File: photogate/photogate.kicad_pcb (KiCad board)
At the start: 2 copper layers, 72.8 x 62.1 mm, 21 parts, among them P2 3poles LOGO, P2 Jack F SJ1-3525N

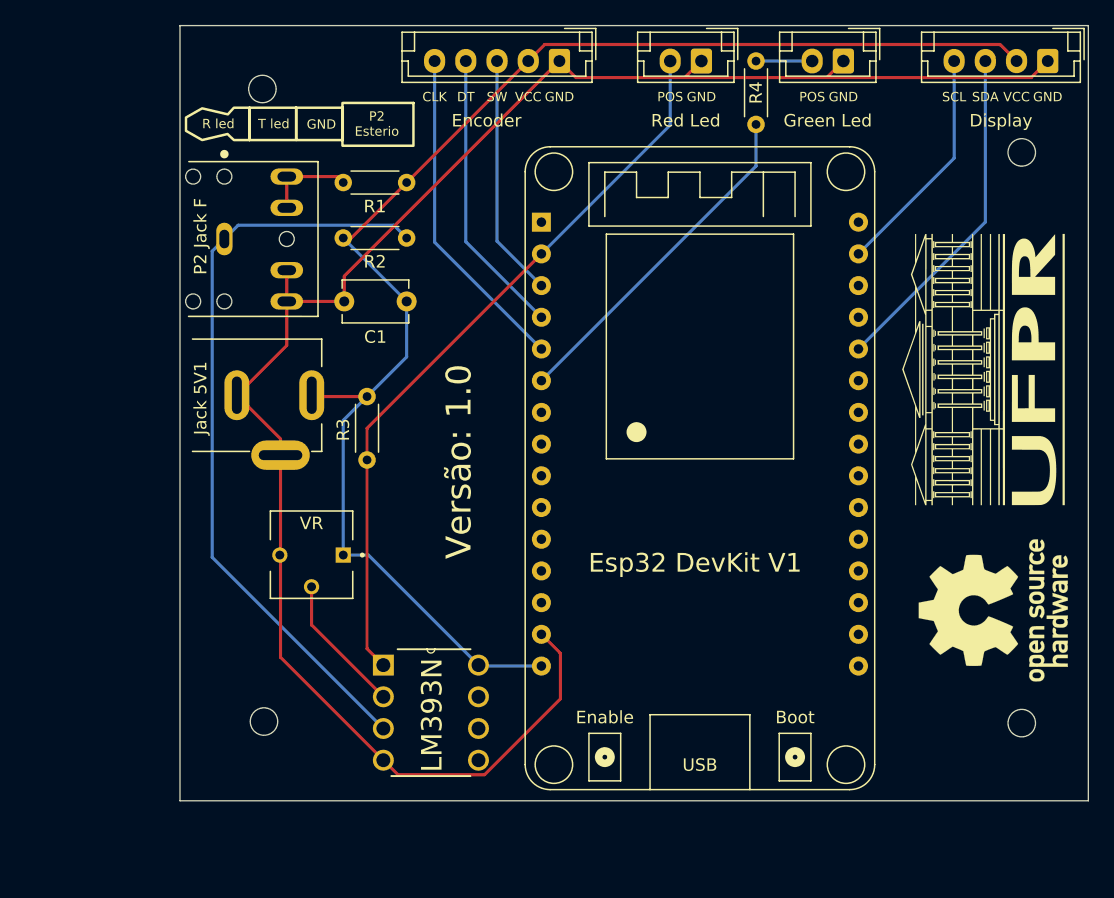
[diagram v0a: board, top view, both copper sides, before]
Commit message: att designe PCB
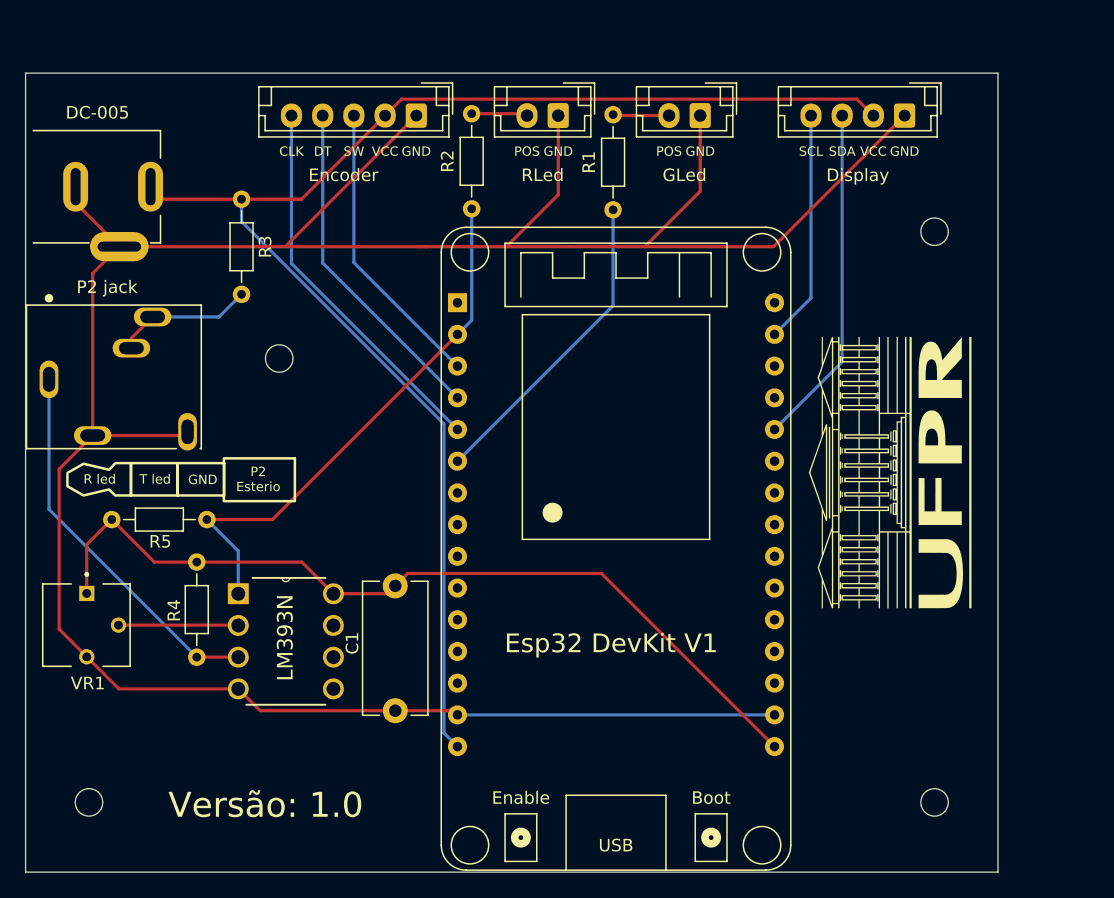
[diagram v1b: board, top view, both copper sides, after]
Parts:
- removed Inferior Esquerdo: MountingHole_2.2mm_M2, MountingHole:MountingHole_2.2mm_M2
- removed P2 Jack F: SJ1-3525N, MyFootprints:CUI_SJ1-3525N
- removed REF** (x3): MountingHole_2.2mm_M2, MountingHole:MountingHole_2.2mm_M2
- removed REF**: OSHW-Logo_11.4x12mm_SilkScreen, Symbol:OSHW-Logo_11.4x12mm_SilkScreen
- added Furo Central: MountingHole_2.2mm_M2, MountingHole:MountingHole_2.2mm_M2, F.Cu at (110.1, 91.4)
- added Furo Inferior1: MountingHole_2.2mm_M2, MountingHole:MountingHole_2.2mm_M2, F.Cu at (94.8, 127.0)
- added Furo Inferior2: MountingHole_2.2mm_M2, MountingHole:MountingHole_2.2mm_M2, F.Cu at (162.6, 127.0)
- added Furo Superior: MountingHole_2.2mm_M2, MountingHole:MountingHole_2.2mm_M2, F.Cu at (162.6, 81.3)
- added P2 jack: SJ1-3515N, MyFootprints:CUI_SJ1-3515N, F.Cu at (91.6, 93.1)
- added R5: 470, Resistor_THT:R_Axial_DIN0204_L3.6mm_D1.6mm_P7.62mm_Horizontal, F.Cu at (104.3, 104.3)
- C1: value 104 -> 104k; footprint Capacitor_THT:C_Disc_D5.1mm_W3.2mm_P5.00mm -> Capacitor_THT:C_Disc_D10.5mm_W5.0mm_P10.00mm
- DC-005: renamed from Jack 5V1
- GLed: renamed from Green Led
- LM393N: value LM393N_A -> LM393N1
- R1: renamed from R4; footprint Resistor_THT:R_Axial_DIN0204_L3.6mm_D1.6mm_P5.08mm_Horizontal -> Resistor_THT:R_Axial_DIN0204_L3.6mm_D1.6mm_P7.62mm_Horizontal
- R2: renamed from R3; footprint Resistor_THT:R_Axial_DIN0204_L3.6mm_D1.6mm_P5.08mm_Horizontal -> Resistor_THT:R_Axial_DIN0204_L3.6mm_D1.6mm_P7.62mm_Horizontal
- R3: renamed from R1; footprint Resistor_THT:R_Axial_DIN0204_L3.6mm_D1.6mm_P5.08mm_Horizontal -> Resistor_THT:R_Axial_DIN0204_L3.6mm_D1.6mm_P7.62mm_Horizontal
- R4: renamed from R2; footprint Resistor_THT:R_Axial_DIN0204_L3.6mm_D1.6mm_P5.08mm_Horizontal -> Resistor_THT:R_Axial_DIN0204_L3.6mm_D1.6mm_P7.62mm_Horizontal
- RLed: renamed from Red Led
- moved P2 3poles 30.0 mm to (102.0, 101.2)
- moved R4 28.5 mm to (103.5, 107.7), turned to -90 degrees
- moved C1 22.8 mm to (119.4, 109.7), turned to -90 degrees
- moved R2 21.8 mm to (125.5, 79.5)
- moved DC-005 21.1 mm to (96.0, 77.7)
- moved VR1 18.9 mm to (94.6, 112.8), turned to -90 degrees
- moved R1 13.3 mm to (136.8, 79.5)
- moved R3 13.3 mm to (107.0, 78.7), turned to -90 degrees
- moved LM393N 12.9 mm to (110.6, 114.8)
- moved GLed 12.3 mm to (143.8, 72.0)
- moved RLed 12.3 mm to (132.4, 72.0)
- moved Encoder 12.3 mm to (121.0, 72.0)
- moved Display 12.3 mm to (160.2, 72.0)
- moved UFPR 11.1 mm to (158.7, 100.8)
- moved Esp32 DevKit V1 9.32 mm to (137.0, 87.0)
- renumbered VR to VR1
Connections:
- DC-005 pad 4: Net-(C1-Pad1) -> Net-(Esp32-Pad15)
- Display pad 2: Net-(C1-Pad1) -> Net-(Esp32-Pad15)
- Encoder pad 2: Net-(C1-Pad1) -> Net-(Esp32-Pad15)
- Esp32 DevKit V1 pad 15: Net-(C1-Pad1) -> Net-(Esp32-Pad15)
- Esp32 DevKit V1 pad 16: unconnected-(Esp32-Pad16) -> Net-(C1-Pad1)
- Esp32 DevKit V1 pad 17: unconnected-(Esp32-Pad17) -> GND
- R2 pad 2: Net-(C1-Pad1) -> Net-(R2-Pad2)
- R3 pad 1: Net-(C1-Pad1) -> Net-(Esp32-Pad15)
- RLed pad 2: /D0 -> Net-(R2-Pad2)
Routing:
- net Net-(Esp32-Pad15): track 0.00 -> 113.2 mm
- net GND: track 143.7 -> 214.2 mm
- net Net-(C1-Pad1): track 114.5 -> 68.7 mm
- net /PHOTODIODE: track 60.8 -> 30.5 mm
- net /D0: track 59.0 -> 43.7 mm
- net Net-(R2-Pad2): track 0.00 -> 4.29 mm
- net /DT: track 23.0 -> 27.1 mm
- net /SW: track 19.5 -> 23.5 mm
- net /CLK: track 26.6 -> 30.7 mm
- net Net-(P2jack1-Pad3): track 7.22 -> 11.1 mm
- net Net-(Esp32-Pad6): track 27.6 -> 25.3 mm
- net Net-(LM393N_A1-Pad2): track 11.2 -> 9.61 mm
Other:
- board size 72.8 x 62.1 mm -> 77.9 x 64 mm
- board text added: "Feito por: Marcio Ap. Bulla Jr. Orientado pelo: Fabiano Yokaichiya Código Fonte: github.com/MarcioBulla/Cronometro-Optico"
- board text removed: "Feito por: Marcio Ap. Bulla Jr. Código Fonte: github.com/MarcioBulla/Cronometro-Optico"
